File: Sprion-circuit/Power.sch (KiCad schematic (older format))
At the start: 31 parts, among them IC1 R3111N211A, IC2 TAR5SB50, J1 Conn_01x03_Female, Q1 IRML6402, Q2 IRML6402, SW1 SSAJ120100, U9 LXDC55FAAA-203

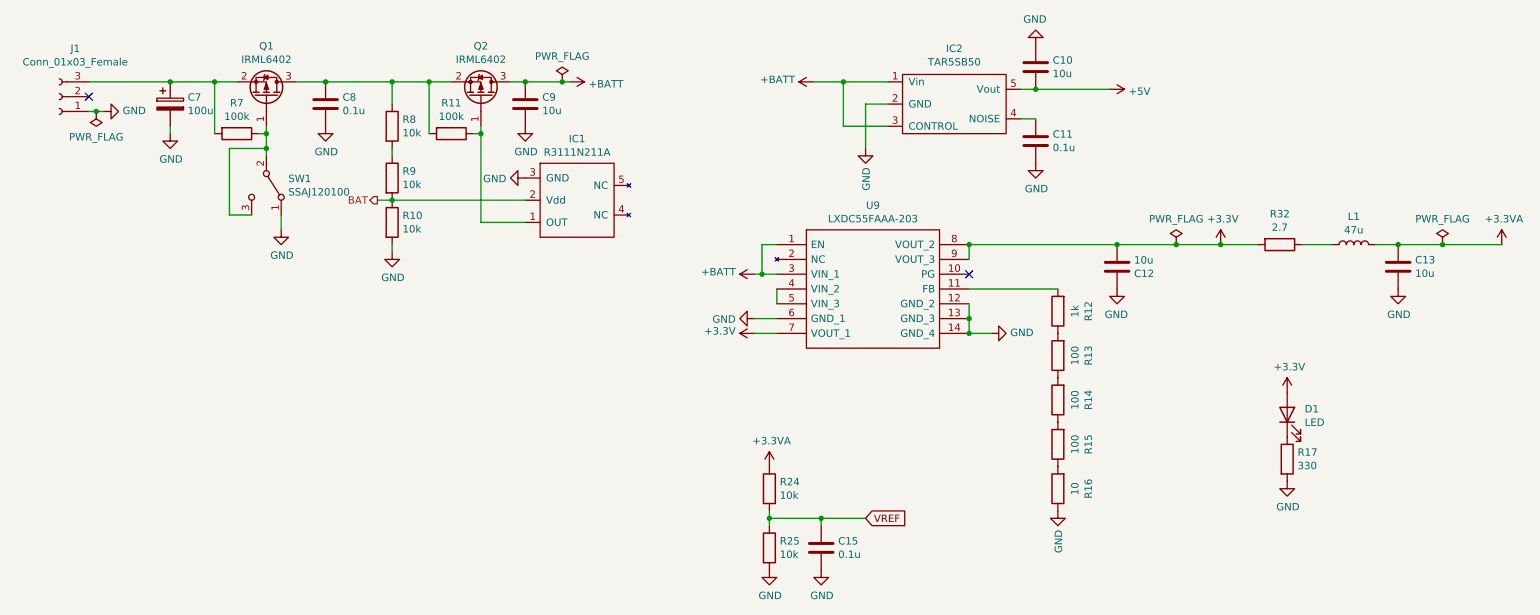
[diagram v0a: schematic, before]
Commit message: add fix feat: でけたー（コミットしてなくてごめん）
ベタ塗、配線、再配置等
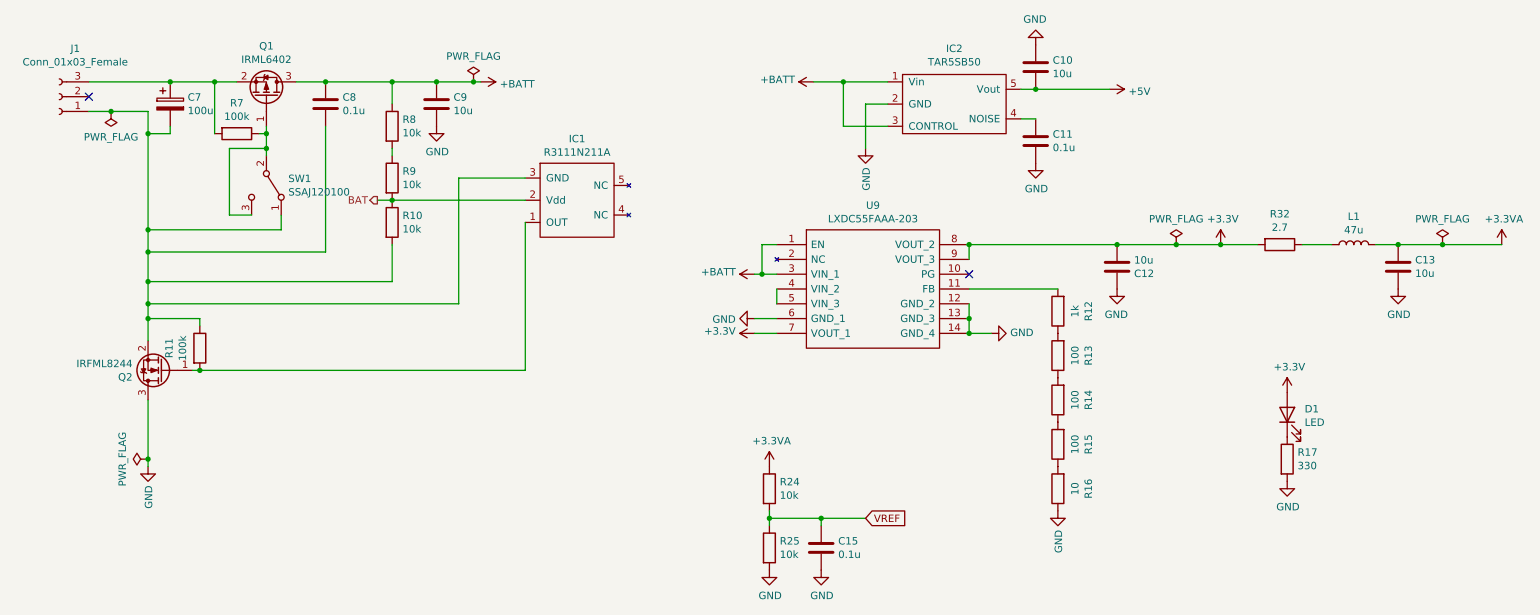
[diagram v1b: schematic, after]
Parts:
- removed Q2: IRML6402, Package_TO_SOT_SMD:SOT-23, symbol Device:Q_PMOS_GSD
- added Q2: IRFML8244, Package_TO_SOT_SMD:SOT-23, symbol Device:Q_NMOS_GSD
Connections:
- net +BATT: now also C8.1, Q1.3 (D), R8.1
- net GND: now also Q2.3 (D); no longer C7.2, C8.2, IC1.3 (GND), J1.1 (Pin_1), R10.2, SW1.1 (A)
- net at R11.1: now also C7.2, C8.2, IC1.3 (GND), J1.1 (Pin_1), R10.2, SW1.1 (A), Q2.2 (S); no longer IC1.1 (OUT)
- new net: IC1.1 (OUT), Q2.1 (G), R11.2
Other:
- moved on the sheet: C9, R11
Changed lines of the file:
@@
 $Descr A4 11693 8268
 encoding utf-8
-Sheet 2 6
+Sheet 6 6
 Title ""
 Date ""
@@
 $EndDescr
 $Comp
-L power:GND #PWR01
-U 1 1 60F3968F
-P 1400 2300
-F 0 "#PWR01" H 1400 2050 50  0001 C CNN
-F 1 "GND" V 1405 2172 50  0000 R CNN
-F 2 "" H 1400 2300 50  0001 C CNN
-F 3 "" H 1400 2300 50  0001 C CNN
-	1    1400 2300
-	0    -1   -1   0
-$EndComp
-$Comp
 L power:PWR_FLAG #FLG01
 U 1 1 60F3A851
-P 1350 2300
-F 0 "#FLG01" H 1350 2375 50  0001 C CNN
-F 1 "PWR_FLAG" H 1350 2473 50  0000 C CNN
-F 2 "" H 1350 2300 50  0001 C CNN
-F 3 "~" H 1350 2300 50  0001 C CNN
-	1    1350 2300
-	-1   0    0    1
-$EndComp
-Wire Wire Line
-	1300 2300 1350 2300
-Wire Wire Line
-	1350 2300 1400 2300
-Connection ~ 1350 2300
+P 1700 4650
+F 0 "#FLG01" H 1700 4725 50  0001 C CNN
+F 1 "PWR_FLAG" H 1700 4823 50  0000 C CNN
+F 2 "" H 1700 4650 50  0001 C CNN
+F 3 "~" H 1700 4650 50  0001 C CNN
+	1    1700 4650
+	0    -1   -1   0
+$EndComp
 $Comp
 L Switch:SW_SPDT SW1
@@
 $EndComp
 $Comp
-L power:GND #PWR03
-U 1 1 60F431E5
-P 2600 3100
-F 0 "#PWR03" H 2600 2850 50  0001 C CNN
-F 1 "GND" H 2605 2927 50  0000 C CNN
-F 2 "" H 2600 3100 50  0001 C CNN
-F 3 "" H 2600 3100 50  0001 C CNN
-	1    2600 3100
-	1    0    0    -1
-$EndComp
-$Comp
 L Device:R R7
 U 1 1 60F43B12
@@
 L power:+BATT #PWR08
 U 1 1 60F46202
-P 4550 2100
-F 0 "#PWR08" H 4550 1950 50  0001 C CNN
-F 1 "+BATT" V 4565 2228 50  0000 L CNN
-F 2 "" H 4550 2100 50  0001 C CNN
-F 3 "" H 4550 2100 50  0001 C CNN
-	1    4550 2100
+P 3950 2100
+F 0 "#PWR08" H 3950 1950 50  0001 C CNN
+F 1 "+BATT" V 3965 2228 50  0000 L CNN
+F 2 "" H 3950 2100 50  0001 C CNN
+F 3 "" H 3950 2100 50  0001 C CNN
+	1    3950 2100
 	0    1    1    0
 $EndComp
@@
 L power:PWR_FLAG #FLG02
 U 1 1 60F505D9
-P 4500 2100
-F 0 "#FLG02" H 4500 2175 50  0001 C CNN
-F 1 "PWR_FLAG" H 4500 2273 50  0000 C CNN
-F 2 "" H 4500 2100 50  0001 C CNN
-F 3 "~" H 4500 2100 50  0001 C CNN
-	1    4500 2100
-	1    0    0    -1
-$EndComp
-$Comp
-L power:GND #PWR07
-U 1 1 60F5182C
-P 4250 2750
-F 0 "#PWR07" H 4250 2500 50  0001 C CNN
-F 1 "GND" V 4255 2622 50  0000 R CNN
-F 2 "" H 4250 2750 50  0001 C CNN
-F 3 "" H 4250 2750 50  0001 C CNN
-	1    4250 2750
-	0    1    1    0
-$EndComp
-Wire Wire Line
-	4550 2100 4500 2100
-Connection ~ 4500 2100
-$Comp
-L power:GND #PWR04
-U 1 1 60F5CE78
-P 2900 2400
-F 0 "#PWR04" H 2900 2150 50  0001 C CNN
-F 1 "GND" H 2905 2227 50  0000 C CNN
-F 2 "" H 2900 2400 50  0001 C CNN
-F 3 "" H 2900 2400 50  0001 C CNN
-	1    2900 2400
-	1    0    0    -1
-$EndComp
+P 3900 2100
+F 0 "#FLG02" H 3900 2175 50  0001 C CNN
+F 1 "PWR_FLAG" H 3900 2273 50  0000 C CNN
+F 2 "" H 3900 2100 50  0001 C CNN
+F 3 "~" H 3900 2100 50  0001 C CNN
+	1    3900 2100
+	1    0    0    -1
+$EndComp
+Wire Wire Line
+	3950 2100 3900 2100
+Connection ~ 3900 2100
 $Comp
 L Device:C C8
@@
 	1    0    0    -1
 $EndComp
-$Comp
-L power:GND #PWR05
-U 1 1 60F66160
-P 3350 3250
-F 0 "#PWR05" H 3350 3000 50  0001 C CNN
-F 1 "GND" H 3355 3077 50  0000 C CNN
-F 2 "" H 3350 3250 50  0001 C CNN
-F 3 "" H 3350 3250 50  0001 C CNN
-	1    3350 3250
-	1    0    0    -1
-$EndComp
-Wire Wire Line
-	3350 3200 3350 3250
 Wire Wire Line
 	2700 2100 2900 2100
 Wire Wire Line
-	3950 2400 3950 2450
-Wire Wire Line
-	3950 3050 4250 3050
-$Comp
-L Device:R R11
-U 1 1 60F7E679
-P 3750 2450
-F 0 "R11" V 3543 2450 50  0000 C CNN
-F 1 "100k" V 3634 2450 50  0000 C CNN
-F 2 "Resistor_SMD:R_0603_1608Metric" V 3680 2450 50  0001 C CNN
-F 3 "~" H 3750 2450 50  0001 C CNN
-	1    3750 2450
-	0    1    1    0
-$EndComp
-Wire Wire Line
-	3900 2450 3950 2450
-Connection ~ 3950 2450
-Wire Wire Line
-	3600 2450 3600 2100
-Connection ~ 3600 2100
-Wire Wire Line
-	3600 2100 3750 2100
-Wire Wire Line
 	3350 2900 4250 2900
-Wire Wire Line
-	3950 2450 3950 3050
 Connection ~ 2900 2100
 Wire Wire Line
@@
 	1850 2100 2150 2100
 Connection ~ 2150 2100
-$Comp
-L power:GND #PWR02
-U 1 1 60F8B6AE
-P 1850 2450
-F 0 "#PWR02" H 1850 2200 50  0001 C CNN
-F 1 "GND" H 1855 2277 50  0000 C CNN
-F 2 "" H 1850 2450 50  0001 C CNN
-F 3 "" H 1850 2450 50  0001 C CNN
-	1    1850 2450
-	1    0    0    -1
-$EndComp
 Wire Wire Line
 	1850 2400 1850 2450
@@
 L Device:C C9
 U 1 1 60F9001F
-P 4250 2250
-F 0 "C9" H 4365 2296 50  0000 L CNN
-F 1 "10u" H 4365 2205 50  0000 L CNN
-F 2 "Capacitor_SMD:C_0603_1608Metric" H 4288 2100 50  0001 C CNN
-F 3 "~" H 4250 2250 50  0001 C CNN
-	1    4250 2250
+P 3650 2250
+F 0 "C9" H 3765 2296 50  0000 L CNN
+F 1 "10u" H 3765 2205 50  0000 L CNN
+F 2 "Capacitor_SMD:C_0603_1608Metric" H 3688 2100 50  0001 C CNN
+F 3 "~" H 3650 2250 50  0001 C CNN
+	1    3650 2250
 	1    0    0    -1
 $EndComp
@@
 L power:GND #PWR06
 U 1 1 60F90B97
-P 4250 2400
-F 0 "#PWR06" H 4250 2150 50  0001 C CNN
-F 1 "GND" H 4255 2227 50  0000 C CNN
-F 2 "" H 4250 2400 50  0001 C CNN
-F 3 "" H 4250 2400 50  0001 C CNN
-	1    4250 2400
-	1    0    0    -1
-$EndComp
-Wire Wire Line
-	4150 2100 4250 2100
-Wire Wire Line
-	4250 2100 4500 2100
-Connection ~ 4250 2100
+P 3650 2400
+F 0 "#PWR06" H 3650 2150 50  0001 C CNN
+F 1 "GND" H 3655 2227 50  0000 C CNN
+F 2 "" H 3650 2400 50  0001 C CNN
+F 3 "" H 3650 2400 50  0001 C CNN
+	1    3650 2400
+	1    0    0    -1
+$EndComp
+Wire Wire Line
+	3650 2100 3900 2100
 $Comp
 L Device:R R8
@@
 Wire Wire Line
 	2900 2100 3350 2100
-Connection ~ 3350 2100
-Wire Wire Line
-	3350 2100 3600 2100
 Wire Wire Line
 	3350 2550 3350 2600
@@
 	0    -1   -1   0
 $EndComp
-$Comp
-L Device:Q_PMOS_GSD Q2
-U 1 1 61B67607
-P 3950 2200
-F 0 "Q2" V 4292 2200 50  0000 C CNN
-F 1 "IRML6402" V 4201 2200 50  0000 C CNN
-F 2 "Package_TO_SOT_SMD:SOT-23" H 4150 2300 50  0001 C CNN
-F 3 "~" H 3950 2200 50  0001 C CNN
-	1    3950 2200
-	0    1    -1   0
-$EndComp
+Wire Wire Line
+	3350 2100 3650 2100
+Connection ~ 3350 2100
+Connection ~ 3650 2100
+$Comp
+L Device:R R11
+U 1 1 60F7E679
+P 2050 3900
+F 0 "R11" V 1843 3900 50  0000 C CNN
+F 1 "100k" V 1934 3900 50  0000 C CNN
+F 2 "Resistor_SMD:R_0603_1608Metric" V 1980 3900 50  0001 C CNN
+F 3 "~" H 2050 3900 50  0001 C CNN
+	1    2050 3900
+	1    0    0    -1
+$EndComp
+$Comp
+L Device:Q_NMOS_GSD Q2
+U 1 1 61B98387
+P 1800 4050
+F 0 "Q2" H 2005 4096 50  0000 L CNN
+F 1 "IRFML8244" H 2005 4005 50  0000 L CNN
+F 2 "Package_TO_SOT_SMD:SOT-23" H 2000 4150 50  0001 C CNN
+F 3 "~" H 1800 4050 50  0001 C CNN
+	1    1800 4050
+	-1   0    0    1
+$EndComp
+Connection ~ 1700 4650
+Wire Wire Line
+	1700 4650 1700 4700
+$Comp
+L power:GND #PWR01
+U 1 1 60F3968F
+P 1700 4700
+F 0 "#PWR01" H 1700 4450 50  0001 C CNN
+F 1 "GND" V 1705 4572 50  0000 R CNN
+F 2 "" H 1700 4700 50  0001 C CNN
+F 3 "" H 1700 4700 50  0001 C CNN
+	1    1700 4700
+	1    0    0    -1
+$EndComp
+Wire Wire Line
+	1700 4250 1700 4650
+Wire Wire Line
+	2000 4050 2050 4050
+Connection ~ 2050 4050
+Wire Wire Line
+	2050 4050 4250 4050
+Wire Wire Line
+	1700 3850 1700 3700
+Wire Wire Line
+	1700 2300 1450 2300
+Wire Wire Line
+	1700 3700 2050 3700
+Wire Wire Line
+	2050 3700 2050 3750
+Connection ~ 1700 3700
+Wire Wire Line
+	1700 2300 1700 2450
+Wire Wire Line
+	4250 3050 4250 4050
+Wire Wire Line
+	3350 3450 1700 3450
+Wire Wire Line
+	3350 3200 3350 3450
+Connection ~ 1700 3450
+Wire Wire Line
+	1700 3450 1700 3600
+Wire Wire Line
+	2600 3100 1700 3100
+Connection ~ 1700 3100
+Wire Wire Line
+	1700 3100 1700 3250
+Wire Wire Line
+	1850 2450 1700 2450
+Connection ~ 1700 2450
+Wire Wire Line
+	1700 2450 1700 3100
+Wire Wire Line
+	2900 2400 2900 3250
+Wire Wire Line
+	2900 3250 1700 3250
+Connection ~ 1700 3250
+Wire Wire Line
+	1700 3250 1700 3450
+Wire Wire Line
+	4250 2750 3800 2750
+Wire Wire Line
+	3800 2750 3800 3600
+Wire Wire Line
+	3800 3600 1700 3600
+Connection ~ 1700 3600
+Wire Wire Line
+	1700 3600 1700 3700
+$Comp
+L power:PWR_FLAG #FLG0101
+U 1 1 61C050C7
+P 1450 2300
+F 0 "#FLG0101" H 1450 2375 50  0001 C CNN
+F 1 "PWR_FLAG" H 1450 2473 50  0000 C CNN
+F 2 "" H 1450 2300 50  0001 C CNN
+F 3 "~" H 1450 2300 50  0001 C CNN
+	1    1450 2300
+	-1   0    0    1
+$EndComp
+Connection ~ 1450 2300
+Wire Wire Line
+	1450 2300 1300 2300
 $EndSCHEMATC
